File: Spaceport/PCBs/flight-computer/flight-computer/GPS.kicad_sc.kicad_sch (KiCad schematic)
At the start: 2 parts, among them U1 SAM-M10Q-00B

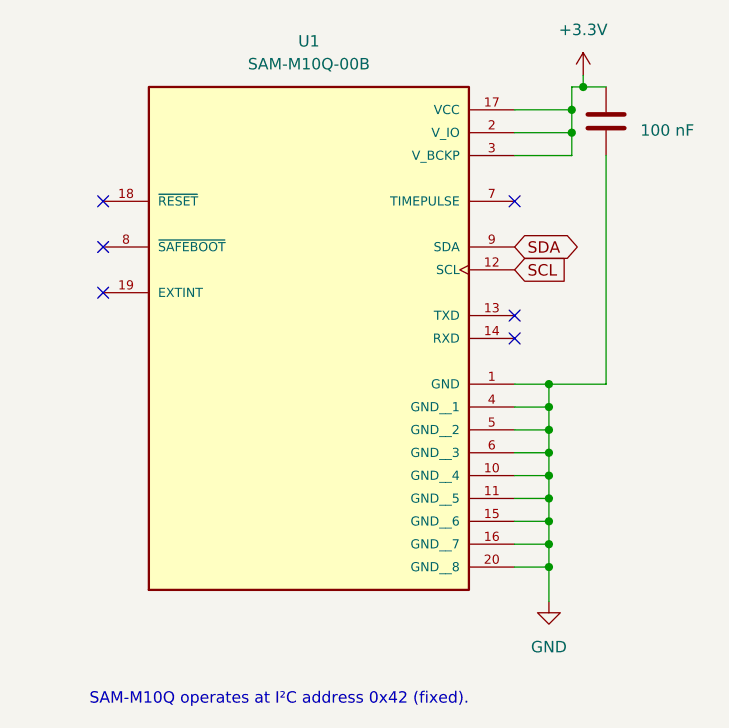
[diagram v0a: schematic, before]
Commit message: added external I2C, SPI, SWD, UART connectors, cleaned up schematics, and changed STM32 schematic for one with power pins. Need to add decoupling capacitors for STM32, external clock for STM32
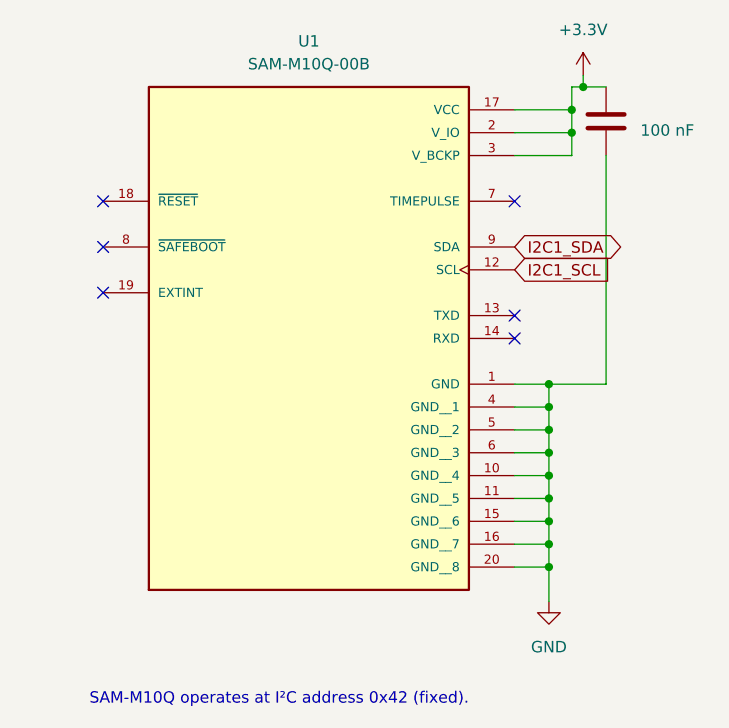
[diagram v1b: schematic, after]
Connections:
- net SCL renamed I2C1_SCL
- net SDA renamed I2C1_SDA
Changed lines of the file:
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@@
 		)
 	)
-	(global_label "SCL"
+	(global_label "I2C1_SCL"
 		(shape input)
 		(at 138.43 82.55 0)
@@
 		)
 		(property "Intersheetrefs" "${INTERSHEET_REFS}"
-			(at 144.9228 82.55 0)
+			(at 150.1842 82.55 0)
 			(effects
 				(font
@@
 		)
 	)
-	(global_label "SDA"
+	(global_label "I2C1_SDA"
 		(shape bidirectional)
 		(at 138.43 80.01 0)
@@
 		)
 		(property "Intersheetrefs" "${INTERSHEET_REFS}"
-			(at 146.0946 80.01 0)
+			(at 151.356 80.01 0)
 			(effects
 				(font
